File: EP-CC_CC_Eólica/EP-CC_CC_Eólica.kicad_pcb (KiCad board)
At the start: 2 copper layers, 19 parts, among them J1 Screw_Terminal_01x03, J2 Screw_Terminal_01x02, Q1 IKW40N120H3, U1 LA100-P, U2 LV25-P

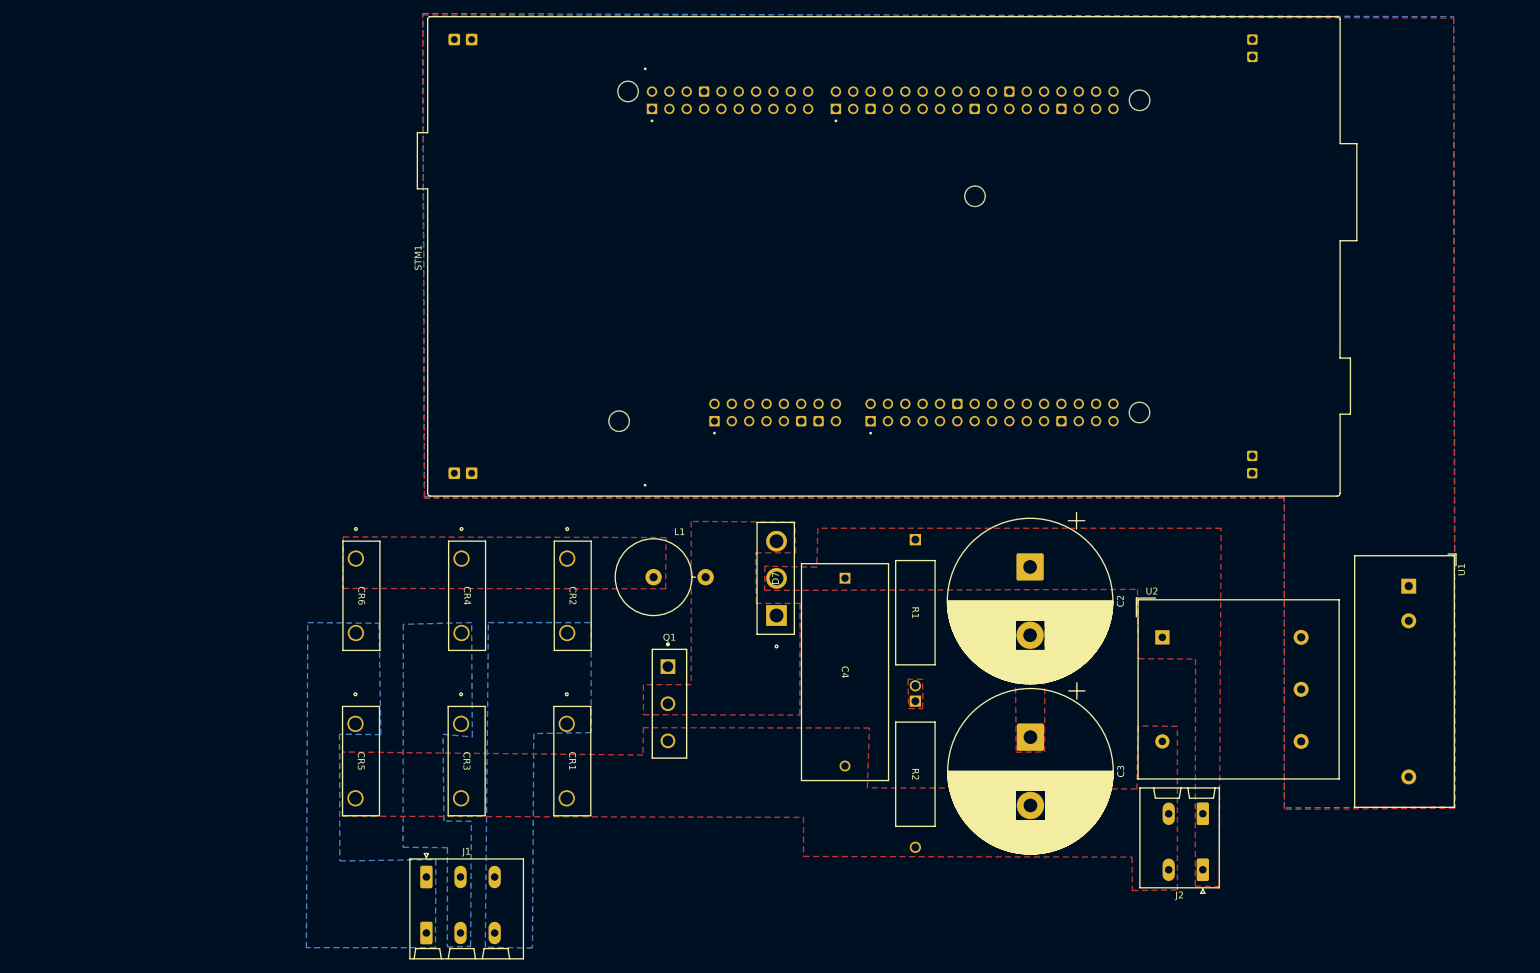
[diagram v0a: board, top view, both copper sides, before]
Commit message: 26/10/19
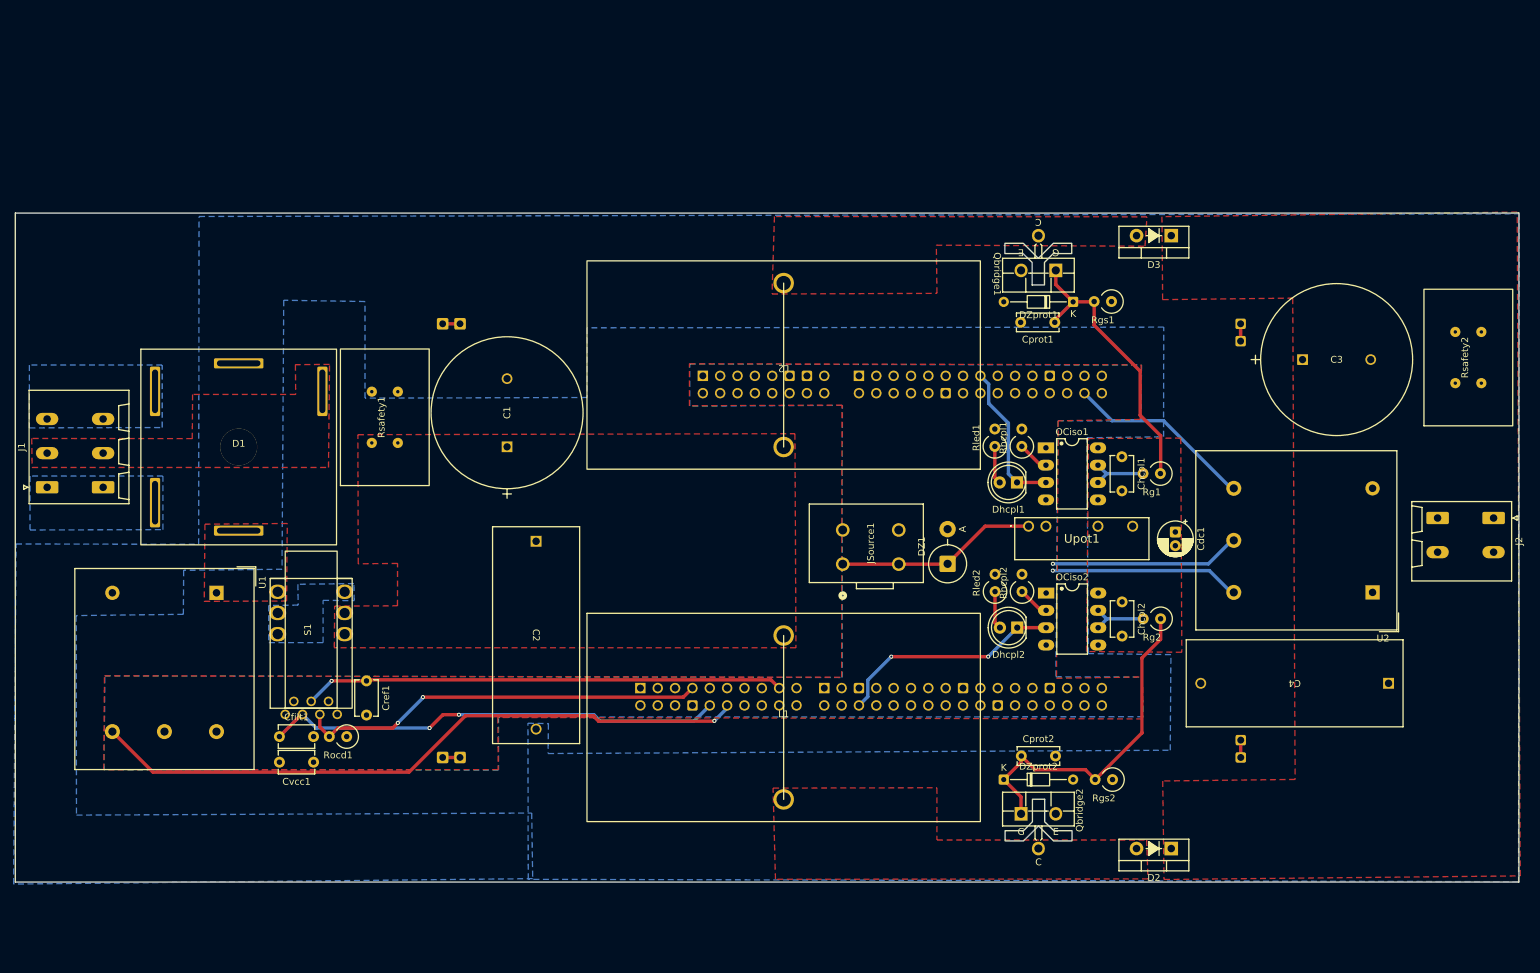
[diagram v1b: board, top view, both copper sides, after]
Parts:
- removed the C3 at (171.7, 128.4)
- removed CR1, CR2, CR3, CR4, CR5, CR6: STBR3012W, Boost:DO-247_STM
- removed D7: C4D20120D, Boost:TO-247-3_CRW
- removed R1, R2: ROX3SJ100K, Boost:RES_ROX3S_TYCO_TYC
- removed the U1 at (227.1, 106.3)
- added C1: 470uF 200V, Boost:CAP_22 X 35_NCH, F.Cu at (95.0, 85.9)
- added C2: 1.5uF 1.3KVDC, Boost:CAP_B32774D1155K000_TDK, F.Cu at (99.3, 99.7)
- added Cdc1: 1uF, Capacitor_THT:CP_Radial_D5.0mm_P2.00mm, F.Cu at (192.9, 98.4)
- added Cfilt1: 47nF - Cer, Capacitor_THT:C_Disc_D5.1mm_W3.2mm_P5.00mm, F.Cu at (61.7, 128.3)
- added Chcpl1: 0.1uF - Cer, Capacitor_THT:C_Disc_D5.1mm_W3.2mm_P5.00mm, F.Cu at (185.1, 87.4)
- added Chcpl2: 0.1uF - Cer, Capacitor_THT:C_Disc_D5.1mm_W3.2mm_P5.00mm, F.Cu at (185.1, 108.6)
- added Cprot1: 10n, Capacitor_THT:C_Disc_D6.0mm_W2.5mm_P5.00mm, F.Cu at (175.2, 67.7)
- added Cprot2: 10n, Capacitor_THT:C_Disc_D6.0mm_W2.5mm_P5.00mm, F.Cu at (170.3, 131.2)
- added Cref1: 47nF - Cer, Capacitor_THT:C_Disc_D5.1mm_W3.2mm_P5.00mm, F.Cu at (74.5, 120.2)
- added Cvcc1: 47nF - Cer, Capacitor_THT:C_Disc_D5.1mm_W3.2mm_P5.00mm, F.Cu at (66.7, 132.1)
- added D1: 600V 35A, Boost:VS-36MT160, F.Cu at (55.8, 86.0)
- added D2: C3D10060A, PCM_Package_TO_SOT_THT_AKL:TO-220-2_Vertical_KA, F.Cu at (192.3, 144.7)
- added D3: C3D10060A, PCM_Package_TO_SOT_THT_AKL:TO-220-2_Vertical_KA, F.Cu at (192.3, 55.0)
- added DZ1: D_Zener_Generic, Diode_THT:D_DO-27_P5.08mm_Vertical_AnodeUp, F.Cu at (159.5, 103.1)
- added DZprot1: 15, Diode_THT:D_DO-34_SOD68_P10.16mm_Horizontal, F.Cu at (177.9, 64.7)
- added DZprot2: 15, Diode_THT:D_DO-34_SOD68_P10.16mm_Horizontal, F.Cu at (167.8, 134.6)
- added Dhcpl1: 1.8V, LED_THT:LED_D5.0mm, F.Cu at (169.7, 91.1)
- added Dhcpl2: 1.8V, LED_THT:LED_D5.0mm, F.Cu at (169.7, 112.4)
- added JSource1: Screw_Terminal_01x02, Boost:CONN2_2604-3102_WAG, F.Cu at (144.2, 103.1)
- added L2: 311uH 15A, Boost:SHBC24W-2R1A0311V, F.Cu at (135.5, 73.9)
- added OCiso1: HCPL-3120, PCM_Package_DIP_AKL:DIP-8_W7.62mm_LongPads, F.Cu at (173.9, 86.1)
- added OCiso2: HCPL-3120, PCM_Package_DIP_AKL:DIP-8_W7.62mm_LongPads, F.Cu at (174.0, 107.3)
- added Qbridge2: 600V40A, Boost:TO-220_High, F.Cu at (172.9, 142.0)
- added Rg1: 22, Resistor_THT:R_Axial_DIN0309_L9.0mm_D3.2mm_P2.54mm_Vertical, F.Cu at (190.7, 89.8)
- added Rg2: 22, Resistor_THT:R_Axial_DIN0309_L9.0mm_D3.2mm_P2.54mm_Vertical, F.Cu at (190.7, 111.1)
- added Rgs1: 10k, Resistor_THT:R_Axial_DIN0309_L9.0mm_D3.2mm_P2.54mm_Vertical, F.Cu at (183.5, 64.7)
- added Rgs2: 10k, Resistor_THT:R_Axial_DIN0309_L9.0mm_D3.2mm_P2.54mm_Vertical, F.Cu at (183.7, 134.6)
- added Rhcpl1: 180, Resistor_THT:R_Axial_DIN0309_L9.0mm_D3.2mm_P2.54mm_Vertical, F.Cu at (170.4, 85.9)
- added Rhcpl2: 180, Resistor_THT:R_Axial_DIN0309_L9.0mm_D3.2mm_P2.54mm_Vertical, F.Cu at (170.4, 107.1)
- added Rled1: 330, Resistor_THT:R_Axial_DIN0309_L9.0mm_D3.2mm_P2.54mm_Vertical, F.Cu at (166.5, 85.9)
- added Rled2: 330, Resistor_THT:R_Axial_DIN0309_L9.0mm_D3.2mm_P2.54mm_Vertical, F.Cu at (166.5, 107.1)
- added Rocd1: 10k, Resistor_THT:R_Axial_DIN0309_L9.0mm_D3.2mm_P2.54mm_Vertical, F.Cu at (71.6, 128.3)
- added Rsafety1: 4.7k, Boost:TWM20J4K7E, F.Cu at (77.1, 81.6)
- added Rsafety2: 4.7k, Boost:TWM20J4K7E, F.Cu at (235.8, 72.8)
- added S1: HE/OL 25A, Boost:HO 25-N_SP33-1000, F.Cu at (66.4, 112.7)
- added U2: LV25-P, Sensor_Voltage:LEM_LV25-P, F.Cu at (221.8, 107.2)
- added Upot1: MEV1S1515SC, Library:MEV1S1505SC, F.Cu at (171.4, 97.5)
- C3: renamed from C2; value C-polar -> 470uF 200V; footprint Capacitor_THT:CP_Radial_D24.0mm_P10.00mm_SnapIn -> Boost:CAP_22 X 35_NCH
- C4: value B32774D1155K000 -> 1.5UF 1.3KVDC
- L1: value L -> 311uH 15A; footprint Inductor_THT:L_Axial_L26.0mm_D11.0mm_P7.62mm_Vertical_Fastron_77A -> Boost:SHBC24W-2R1A0311V
- Qbridge1: renamed from Q1; value IKW40N120H3 -> 600V40A; footprint Boost:INF-PG-TO247-3 -> Boost:TO-220_High
- STM1: moved to B.Cu
- moved U1 138.7 mm to (52.5, 107.3), turned to -90 degrees
- moved Qbridge1 85.2 mm to (172.8, 57.8), turned to 180 degrees
- moved C4 81.1 mm to (224.1, 120.5), turned to 180 degrees
- moved J1 79.6 mm to (27.7, 91.8), turned to 90 degrees
- moved J2 66.8 mm to (239.5, 96.3), turned to -90 degrees
- moved C3 50.1 mm to (211.5, 73.2), turned to 0 degrees
- moved L1 28.0 mm to (135.5, 125.5)
- moved STM1 21.9 mm to (113.6, 67.9), turned to -90 degrees
- renumbered U2 to U1
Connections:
- net 3V3 renamed +3.3V
- C3 pad 2: /CAP_MID -> Earth
- J2 pad 1: /BOOST+ -> Earth
- J2 pad 2: Earth -> /BOOST+
- L1 pad 1: /RECT+ -> /L+
- L1 pad 2: /IGBT+ -> /IGBT1+
- Qbridge1 pad 1: STM_IGBT -> S1
- Qbridge1 pad 2: /IGBT+ -> /IGBT2+
- STM1 pad PA4: unconnected-(STM1-PadPA4) -> STM_Vref
- STM1 pad PA5: unconnected-(STM1-PadPA5) -> STM_Iin
- STM1 pad PA6: unconnected-(STM1-PadPA6) -> STM_Vin
- STM1 pad PB12: unconnected-(STM1-PadPB12) -> STM_OCD
- STM1 pad PE11: unconnected-(STM1-PadPE11) -> STM_S2
- STM1 pad PE9: unconnected-(STM1-PadPE9) -> STM_S1
- STM1 pad PF9: unconnected-(STM1-PadPF9) -> STM_Vout
- U1 pad 1: /BOOST+ -> /RECT+
- U1 pad 4: STM_V -> STM_Vin
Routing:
- net STM_Vin: track 0.00 -> 97.4 mm, vias 0 -> 1
- net STM_Vref: track 0.00 -> 70.3 mm, vias 0 -> 1
- net STM_Iin: track 0.00 -> 67.3 mm, vias 0 -> 2
- net STM_OCD: track 0.00 -> 60.0 mm, vias 0 -> 2
- net S2: track 0.00 -> 50.4 mm
- net S1: track 0.00 -> 42.1 mm
- net GND: track 0.00 -> 37.8 mm, vias 0 -> 1
- net STM_S2: track 0.00 -> 33.5 mm, vias 0 -> 2
- net 15V: track 0.00 -> 29.5 mm
- net +3.3V: track 0.00 -> 27.6 mm, vias 0 -> 1
- net STM_Vout: track 0.00 -> 27.3 mm
- net STM_S1: track 0.00 -> 22.1 mm
- net /V1: track 0.00 -> 8.96 mm
- net /V2: track 0.00 -> 8.88 mm
- net /Vled1: track 0.00 -> 5.57 mm
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- added copper zone on F.Cu, net /FAN_B
- added copper zone on F.Cu, net /IGBT1+
- added copper zone on F.Cu, net /IGBT2+
- added copper zone on F.Cu, net /L+
- added copper zone on B.Cu, net /Winding
- added copper zone on B.Cu, net Earth
- added copper zone on F.Cu, net Vcc_Pot
- removed copper zone on F.Cu, net /CAP_MID
- removed copper zone on B.Cu, net /FAN_B
- removed copper zone on F.Cu, net /IGBT+
- removed copper zone on F.Cu, net /R_MID
- removed copper zone on F.Cu, net Earth
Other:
- board outline added: 220.1 x 98 mm
